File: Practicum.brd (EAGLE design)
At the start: 40.6 x 26.3 mm, 14 parts, among them U1 ATMEGA328P-AU

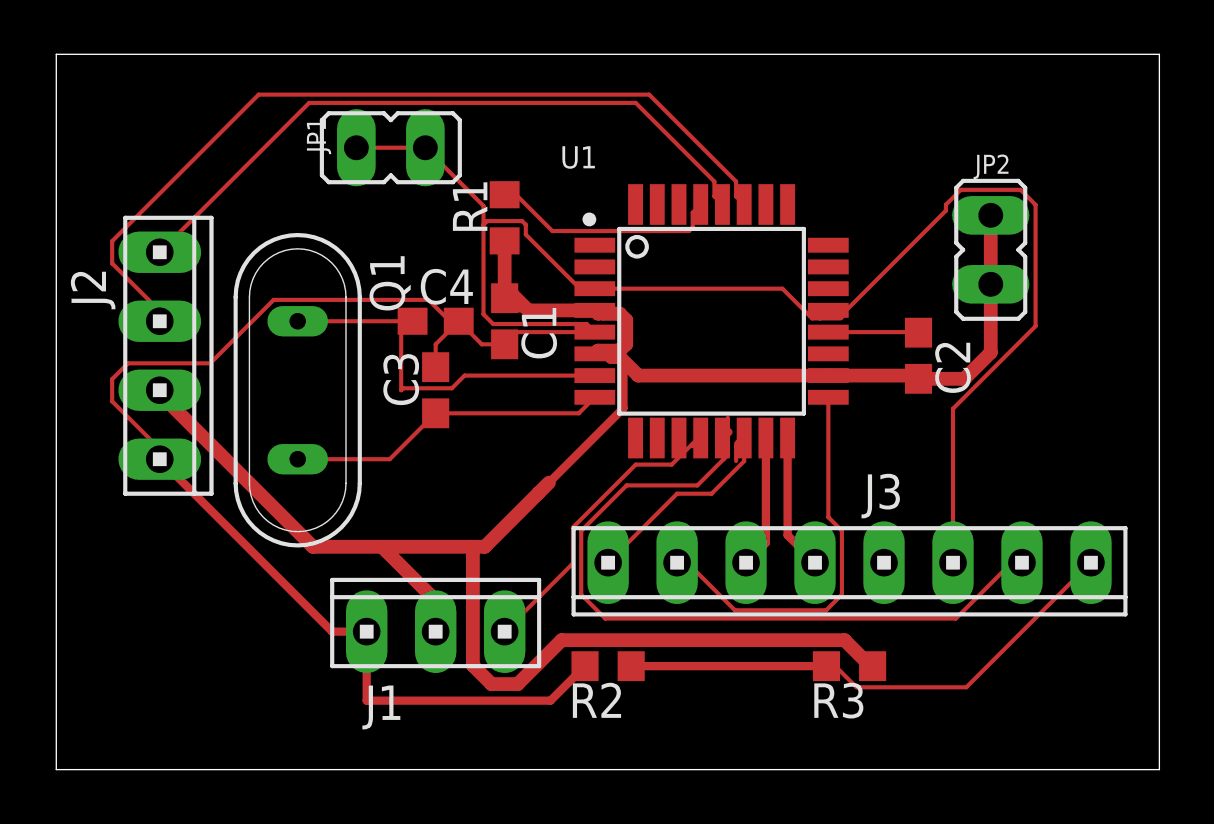
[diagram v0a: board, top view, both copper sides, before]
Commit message: Add files via upload
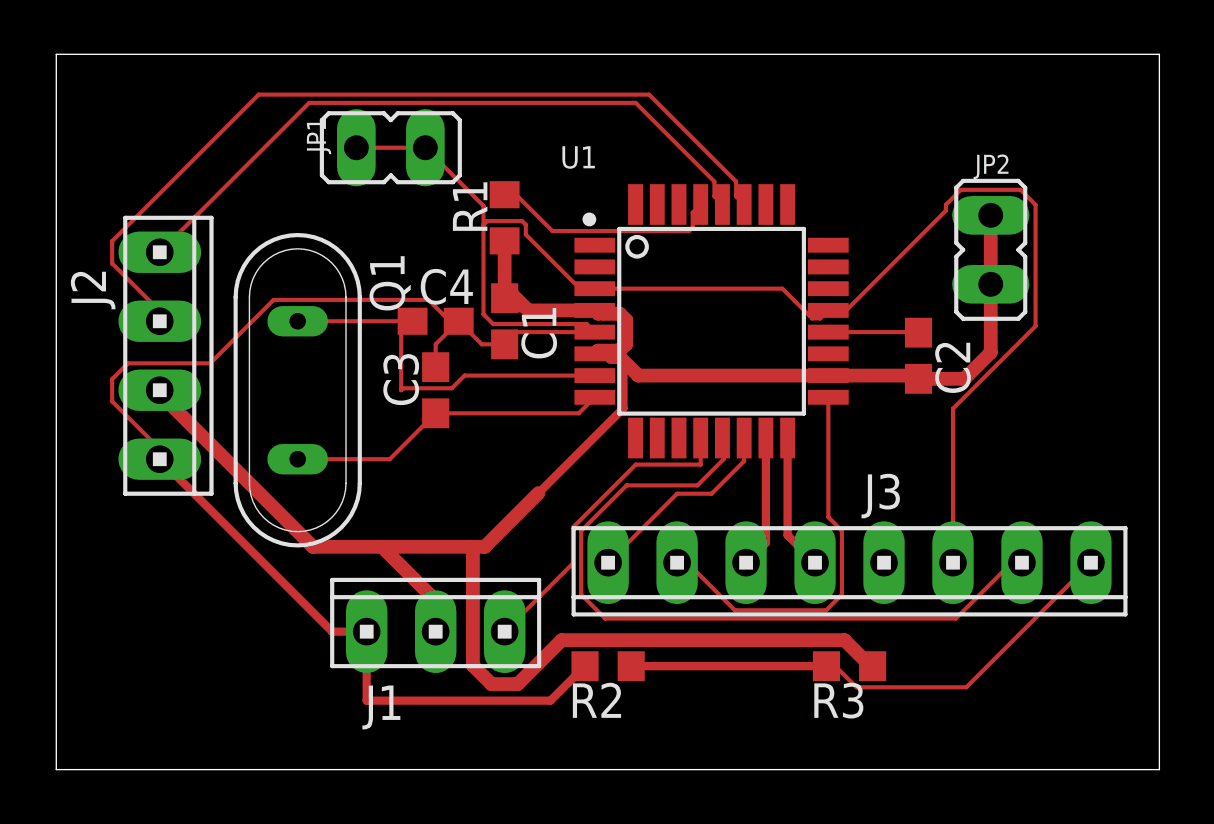
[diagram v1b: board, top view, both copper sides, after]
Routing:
- net N$8: track 28.9 -> 27.0 mm
- net VCC: track 87.4 -> 85.7 mm
- net N$12: track 8.38 -> 7.41 mm
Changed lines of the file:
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@@
 <drawing>
 <settings>
-<setting alwaysvectorfont="yes"/>
+<setting alwaysvectorfont="no"/>
 <setting verticaltext="up"/>
 </settings>
@@
 <contactref element="U1" pad="29"/>
 <contactref element="R1" pad="2"/>
-<wire x1="16.93" y1="21.59" x2="16.72" y2="21.38" width="0.1524" layer="1"/>
 <wire x1="16.72" y1="21.38" x2="16.51" y2="21.17" width="0.1524" layer="1"/>
 <wire x1="23.4336" y1="19.9653125" x2="23.2996875" y2="19.8314" width="0.1524" layer="1"/>
@@
 <wire x1="18.2" y1="2.54" x2="11.43" y2="2.54" width="0.3048" layer="1"/>
 <wire x1="11.43" y1="2.54" x2="11.43" y2="5.08" width="0.3048" layer="1"/>
-<wire x1="28.86585" y1="16.6898" x2="28.1336" y2="16.6898" width="0.3048" layer="1"/>
 <wire x1="2.0574" y1="13.559675" x2="2.0574" y2="14.380325" width="0.1524" layer="1"/>
 <wire x1="2.0574" y1="14.380325" x2="2.637675" y2="14.9606" width="0.1524" layer="1"/>
@@
 <wire x1="33.02" y1="13.2875" x2="36.061" y2="16.3285" width="0.1524" layer="1"/>
 <wire x1="32.759" y1="20.79928125" x2="32.759" y2="20.58295" width="0.1524" layer="1"/>
-<wire x1="32.759" y1="20.58295" x2="28.86585" y2="16.6898" width="0.1524" layer="1"/>
-<wire x1="28.43" y1="16.91" x2="28.1336" y2="16.6898" width="0" layer="19" extent="1-1"/>
+<wire x1="32.759" y1="20.58295" x2="28.948025" y2="16.771975" width="0.1524" layer="1"/>
+<wire x1="28.43" y1="16.91" x2="28.81" y2="16.91" width="0.1524" layer="1"/>
+<wire x1="28.81" y1="16.91" x2="28.948025" y2="16.771975" width="0.1524" layer="1"/>
 </signal>
 <signal name="VCC">
@@
 <wire x1="20.6746875" y1="15.6064" x2="20.6164" y2="15.6064" width="0.1524" layer="1"/>
 <wire x1="20.6164" y1="15.6064" x2="20.32" y2="15.31" width="0.1524" layer="1"/>
-<wire x1="31.75" y1="13.97" x2="31.75" y2="14.39" width="0.1524" layer="1"/>
 <wire x1="34.41" y1="17.87" x2="34.41" y2="15.36" width="0.508" layer="1"/>
 <wire x1="33.44" y1="14.39" x2="31.75" y2="14.39" width="0.508" layer="1"/>
@@
 <contactref element="J1" pad="2"/>
 <contactref element="R3" pad="1"/>
-<wire x1="3.81" y1="13.97" x2="4.56988125" y2="13.97" width="0.3048" layer="1"/>
 <wire x1="20.7483375" y1="15.1914" x2="20.7483375" y2="15.4286" width="0.3048" layer="1"/>
 <wire x1="13.97" y1="5.08" x2="13.97" y2="6.22436875" width="0.508" layer="1"/>
@@
 <wire x1="3.81" y1="13.84436875" x2="3.81" y2="13.97" width="0.508" layer="1"/>
 <wire x1="3.81" y1="13.84436875" x2="9.4488" y2="8.20556875" width="0.508" layer="1"/>
-<wire x1="18.14245" y1="10.5664" x2="17.758025" y2="10.181975" width="0.508" layer="1"/>
 <wire x1="17.758025" y1="10.181975" x2="15.78161875" y2="8.20556875" width="0.508" layer="1"/>
 <wire x1="15.78161875" y1="8.20556875" x2="15.24" y2="8.20556875" width="0.508" layer="1"/>
@@
 <contactref element="J1" pad="1"/>
 <contactref element="U1" pad="12"/>
-<wire x1="23.4336" y1="11.9136" x2="23.73" y2="12.21" width="0.1524" layer="1"/>
-<wire x1="23.64" y1="12.21" x2="23.73" y2="12.21" width="0.1524" layer="1"/>
-<wire x1="22.6614" y1="11.2314" x2="23.64" y2="12.21" width="0.1524" layer="1"/>
-<wire x1="21.33741875" y1="11.2314" x2="22.6614" y2="11.2314" width="0.1524" layer="1"/>
+<wire x1="23.73" y1="12.21" x2="23.73" y2="11.2314" width="0.1524" layer="1"/>
+<wire x1="21.33741875" y1="11.2314" x2="23.73" y2="11.2314" width="0.1524" layer="1"/>
 <wire x1="19.0246" y1="8.91858125" x2="21.33741875" y2="11.2314" width="0.1524" layer="1"/>
 <wire x1="19.0246" y1="7.5946" x2="19.0246" y2="8.91858125" width="0.1524" layer="1"/>
@@
 <contactref element="R2" pad="1"/>
 <contactref element="J3" pad="8"/>
-<wire x1="28.57895" y1="3.81" x2="28.36" y2="3.81" width="0.3048" layer="1"/>
 <wire x1="28.36" y1="3.81" x2="27.94" y2="3.81" width="0.3048" layer="1"/>
 <wire x1="27.94" y1="3.81" x2="21.17" y2="3.81" width="0.3048" layer="1"/>
@@
 <contactref element="J3" pad="1"/>
 <contactref element="U1" pad="14"/>
-<wire x1="25.1098" y1="11.9898" x2="25.33" y2="12.21" width="0.3048" layer="1"/>
-<wire x1="25.0336" y1="11.3653125" x2="25.0336" y2="11.9136" width="0.1524" layer="1"/>
-<wire x1="25.0336" y1="11.9136" x2="25.1098" y2="11.9898" width="0.1524" layer="1"/>
 <wire x1="20.32" y1="7.62" x2="22.86" y2="10.16" width="0.1524" layer="1"/>
 <wire x1="22.86" y1="10.16" x2="24.13" y2="10.16" width="0.1524" layer="1"/>
@@
 <contactref element="J3" pad="7"/>
 <contactref element="U1" pad="13"/>
-<wire x1="24.7502" y1="12.4302" x2="24.575" y2="12.255" width="0.3048" layer="1"/>
 <wire x1="24.575" y1="12.255" x2="24.53" y2="12.21" width="0.3048" layer="1"/>
 <wire x1="24.575" y1="11.43" x2="24.575" y2="12.255" width="0.1524" layer="1"/>
-<wire x1="24.7288" y1="11.5838" x2="24.575" y2="11.43" width="0.1524" layer="1"/>
-<wire x1="24.7288" y1="12.9570875" x2="24.7288" y2="11.5838" width="0.1524" layer="1"/>
 <wire x1="19.3294" y1="6.447675" x2="19.3294" y2="8.792325" width="0.1524" layer="1"/>
 <wire x1="35.56" y1="7.62" x2="35.182925" y2="7.62" width="0.1524" layer="1"/>
